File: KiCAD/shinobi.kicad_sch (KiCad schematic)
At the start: 111 parts, among them J1 61300211121, J2 217179-0001, J3 61301011121, J4 61300711121, Q1 PUMH13-QF, U1 TPS62825DMQR, U2 TPS62825DMQR, U3 CH343P, U4 ESP8285, U5 74LVC2G17GW-Q100H, U6 SI5351A, U7 TV5725, U8 W9864G2JH-6, Y1 26MHz 10pF 2520, Y2 25MHz 10pF 2520, Y3 27MHz 10pF 2520

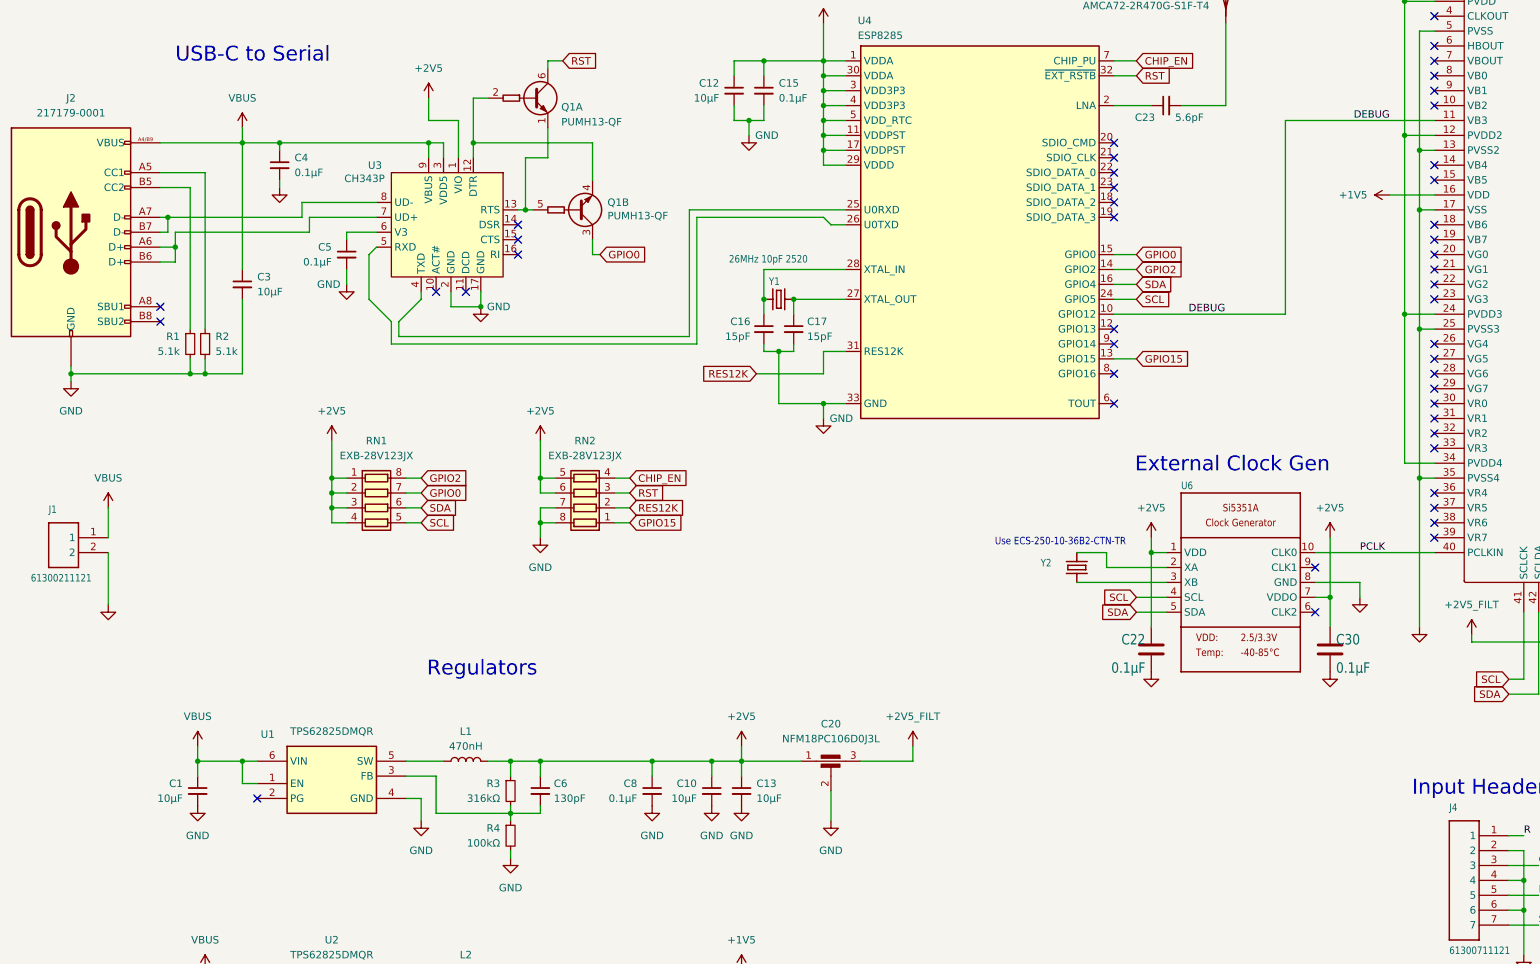
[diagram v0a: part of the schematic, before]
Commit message: small updates
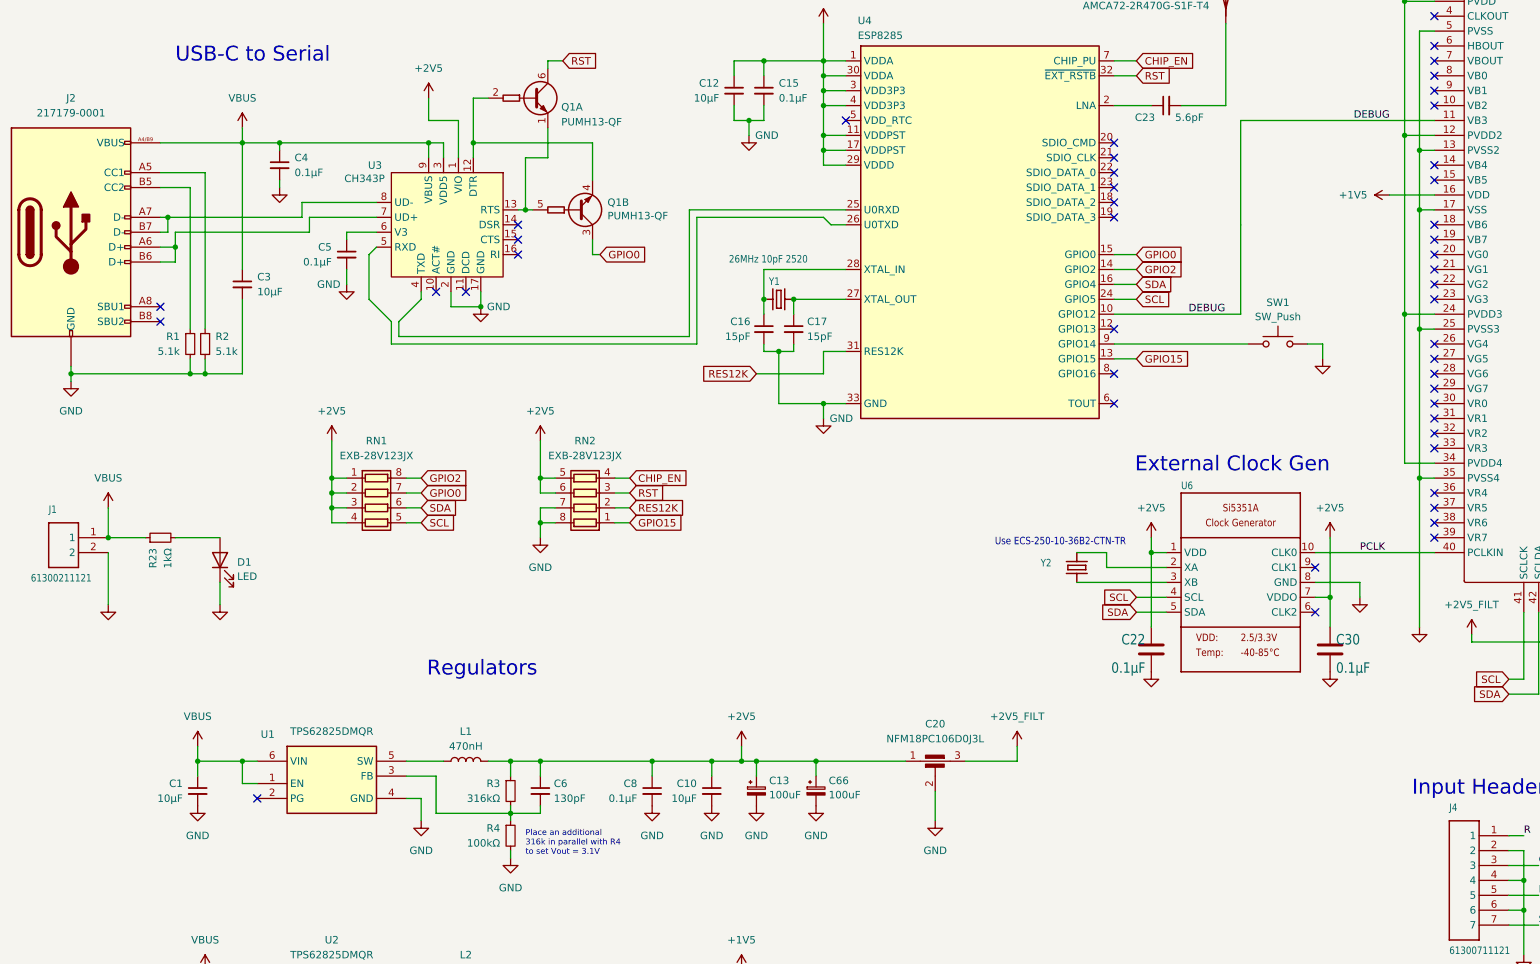
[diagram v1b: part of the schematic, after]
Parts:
- removed C13: 10μF, Capacitor_SMD:C_0603_1608Metric, symbol Device:C_Small
- added C13, C66: 100uF, Capacitor_Tantalum_SMD:CP_EIA-2012-12_Kemet-R, symbol Device:C_Polarized_Small
- added D1: LED, LED_SMD:LED_0603_1608Metric, symbol Device:LED
- added R23: 1kΩ, Resistor_SMD:R_0402_1005Metric, symbol Device:R_Small
- added SW1: SW_Push, Button_Switch_SMD:SW_SPST_B3U-1000P, symbol Switch:SW_Push
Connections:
- net +2V5: now also C13.1, C66.1; no longer U4.5 (VDD_RTC)
- net GND: now also C13.2, C66.2, D1.1 (K), SW1.2
- net VBUS: now also R23.1
- net at U4.9 (GPIO14): now also SW1.1
- new net: D1.2 (A), R23.2
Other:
- note added: "Place an additional 316k in parallel with R4 to set Vout = 3.1V"
- moved on the sheet: C20

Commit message: updating files
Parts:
- C23: renamed from C22; symbol Device:C -> Device:C_Small
- C31: renamed from C30; symbol Device:C -> Device:C_Small
- C32: renamed from C31; symbol Device:C -> Device:C_Small
- C33: renamed from C32; symbol Device:C -> Device:C_Small
- C37: renamed from C36; symbol Device:C -> Device:C_Small
- C39: renamed from C38; symbol Device:C -> Device:C_Small
- C40: renamed from C39; symbol Device:C -> Device:C_Small
- C41: renamed from C40; symbol Device:C -> Device:C_Small
- C42: renamed from C41; symbol Device:C -> Device:C_Small
- C43: renamed from C42; symbol Device:C -> Device:C_Small
- C44: renamed from C43; symbol Device:C -> Device:C_Small
- C45: renamed from C44; symbol Device:C -> Device:C_Small
- C46: renamed from C45; symbol Device:C -> Device:C_Small
- C47: renamed from C46; symbol Device:C -> Device:C_Small
- C48: renamed from C47; symbol Device:C -> Device:C_Small
- C49: renamed from C48; symbol Device:C -> Device:C_Small
- C50: renamed from C49; symbol Device:C -> Device:C_Small
- C51: renamed from C50; symbol Device:C -> Device:C_Small
- C52: renamed from C51; symbol Device:C -> Device:C_Small
- C53: renamed from C52; symbol Device:C -> Device:C_Small
- C54: renamed from C53; symbol Device:C -> Device:C_Small
- C55: renamed from C54; symbol Device:C -> Device:C_Small
- C56: renamed from C55; symbol Device:C -> Device:C_Small
- C57: renamed from C56; symbol Device:C -> Device:C_Small
- C58: renamed from C57; symbol Device:C -> Device:C_Small
- C59: renamed from C58; symbol Device:C -> Device:C_Small
- C60: renamed from C59; symbol Device:C -> Device:C_Small
- C61: renamed from C60; symbol Device:C -> Device:C_Small
- C62: renamed from C61; symbol Device:C -> Device:C_Small
- C63: renamed from C62; symbol Device:C -> Device:C_Small
- C64: renamed from C63; symbol Device:C -> Device:C_Small
- C65: renamed from C64; symbol Device:C -> Device:C_Small
- C66: renamed from C65; symbol Device:C -> Device:C_Small
- D1: value LED -> green
- SW1: value SW_Push -> B3U-1000P
- renumbered C14 to C13, C13 to C14, C66 to C20, C20 to C22, C23 to C24, C24 to C25, C25 to C26, C26 to C27, C27 to C28, C28 to C29, C29 to C30, C33 to C34, C34 to C35, C35 to C36, C37 to C38, R23 to R1, R9 to R10, R10 to R11, R11 to R12, R12 to R13, R13 to R14, R14 to R15, R15 to R16, R16 to R17, R17 to R18, R18 to R19, R1 to R2, R19 to R20, R20 to R21, R21 to R22, R22 to R23, R2 to R3, R3 to R4, R4 to R5, R5 to R6, R6 to R7, R7 to R8, R8 to R9
